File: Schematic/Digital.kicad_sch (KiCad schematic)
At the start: 19 parts, among them U801 74HC165, U802 74HC165, U803 74HC165, U804 74HC165, U805 74HC595, U806 ESP32-S3-DevKitC, U808 MCP42010, U809 MCP42010, U810 MCP42010, U811 MCP42010

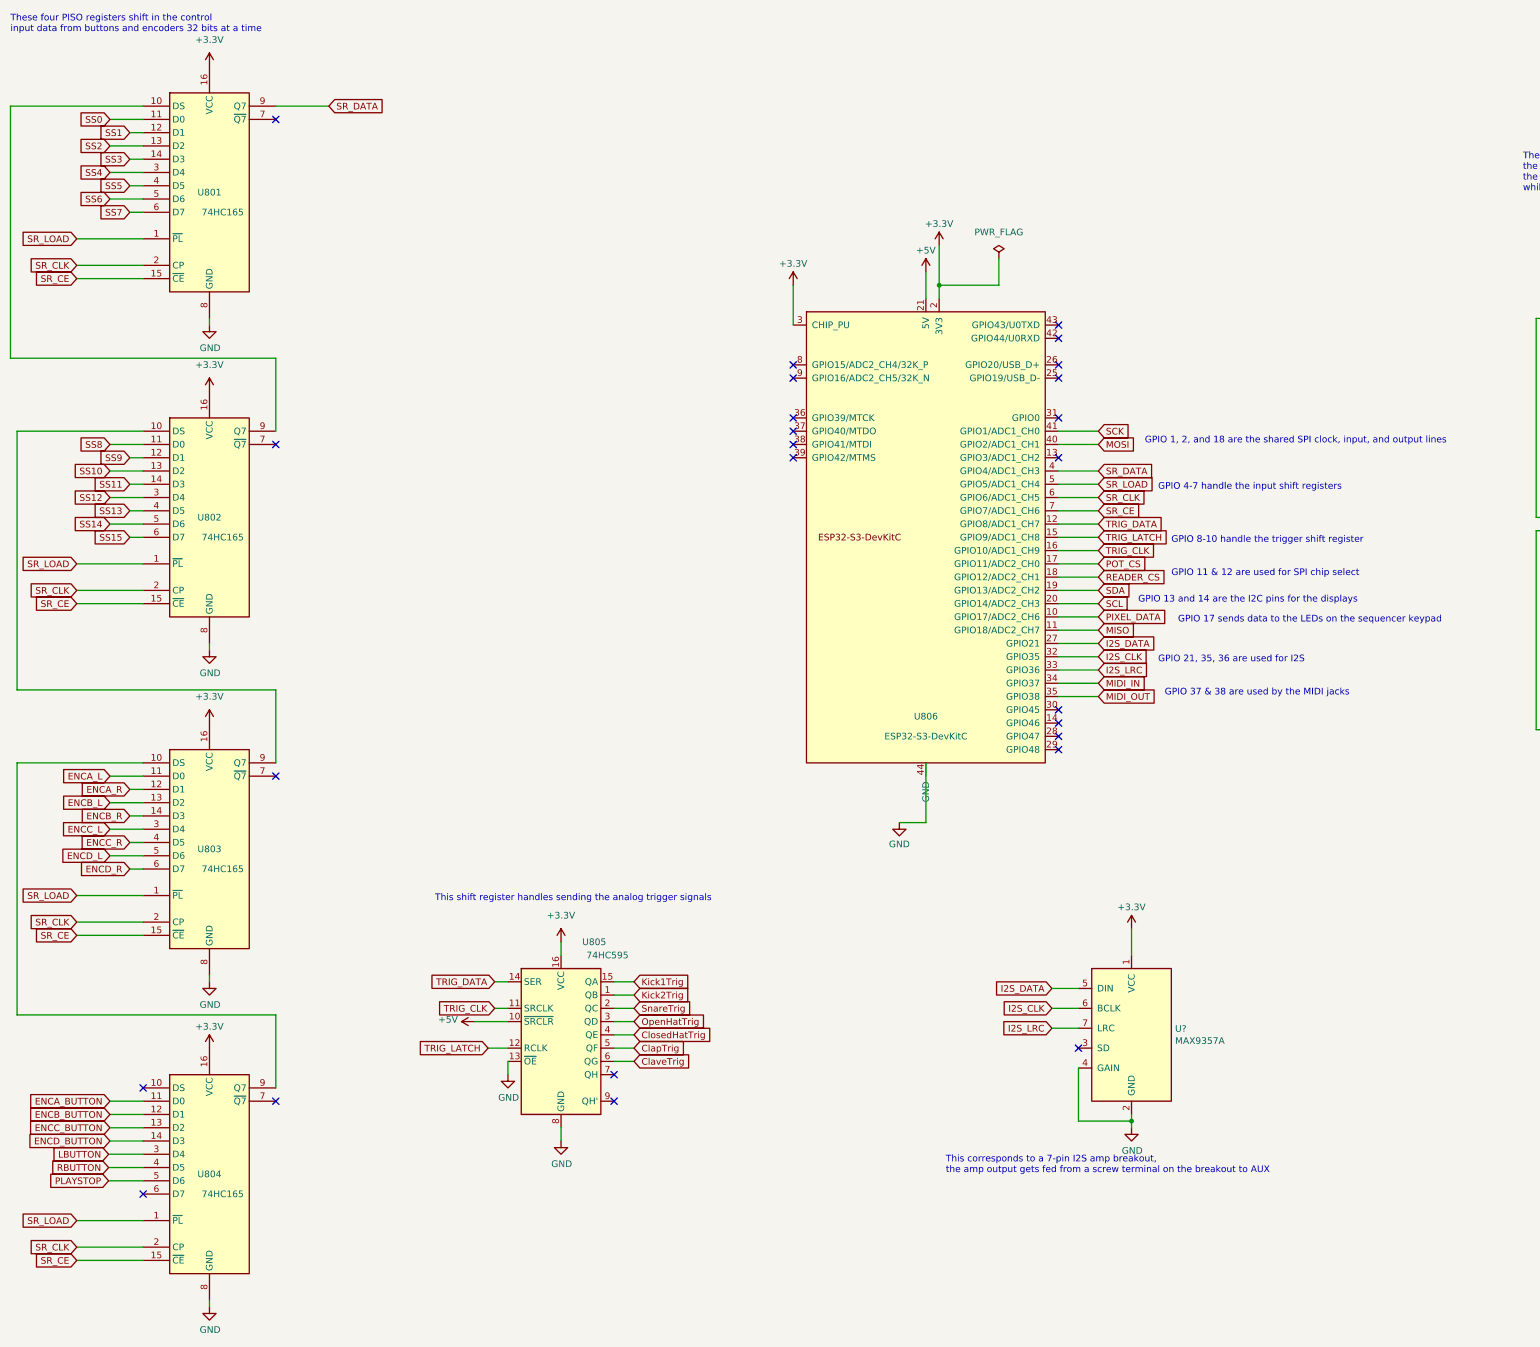
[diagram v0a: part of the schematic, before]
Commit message: cleansing fire
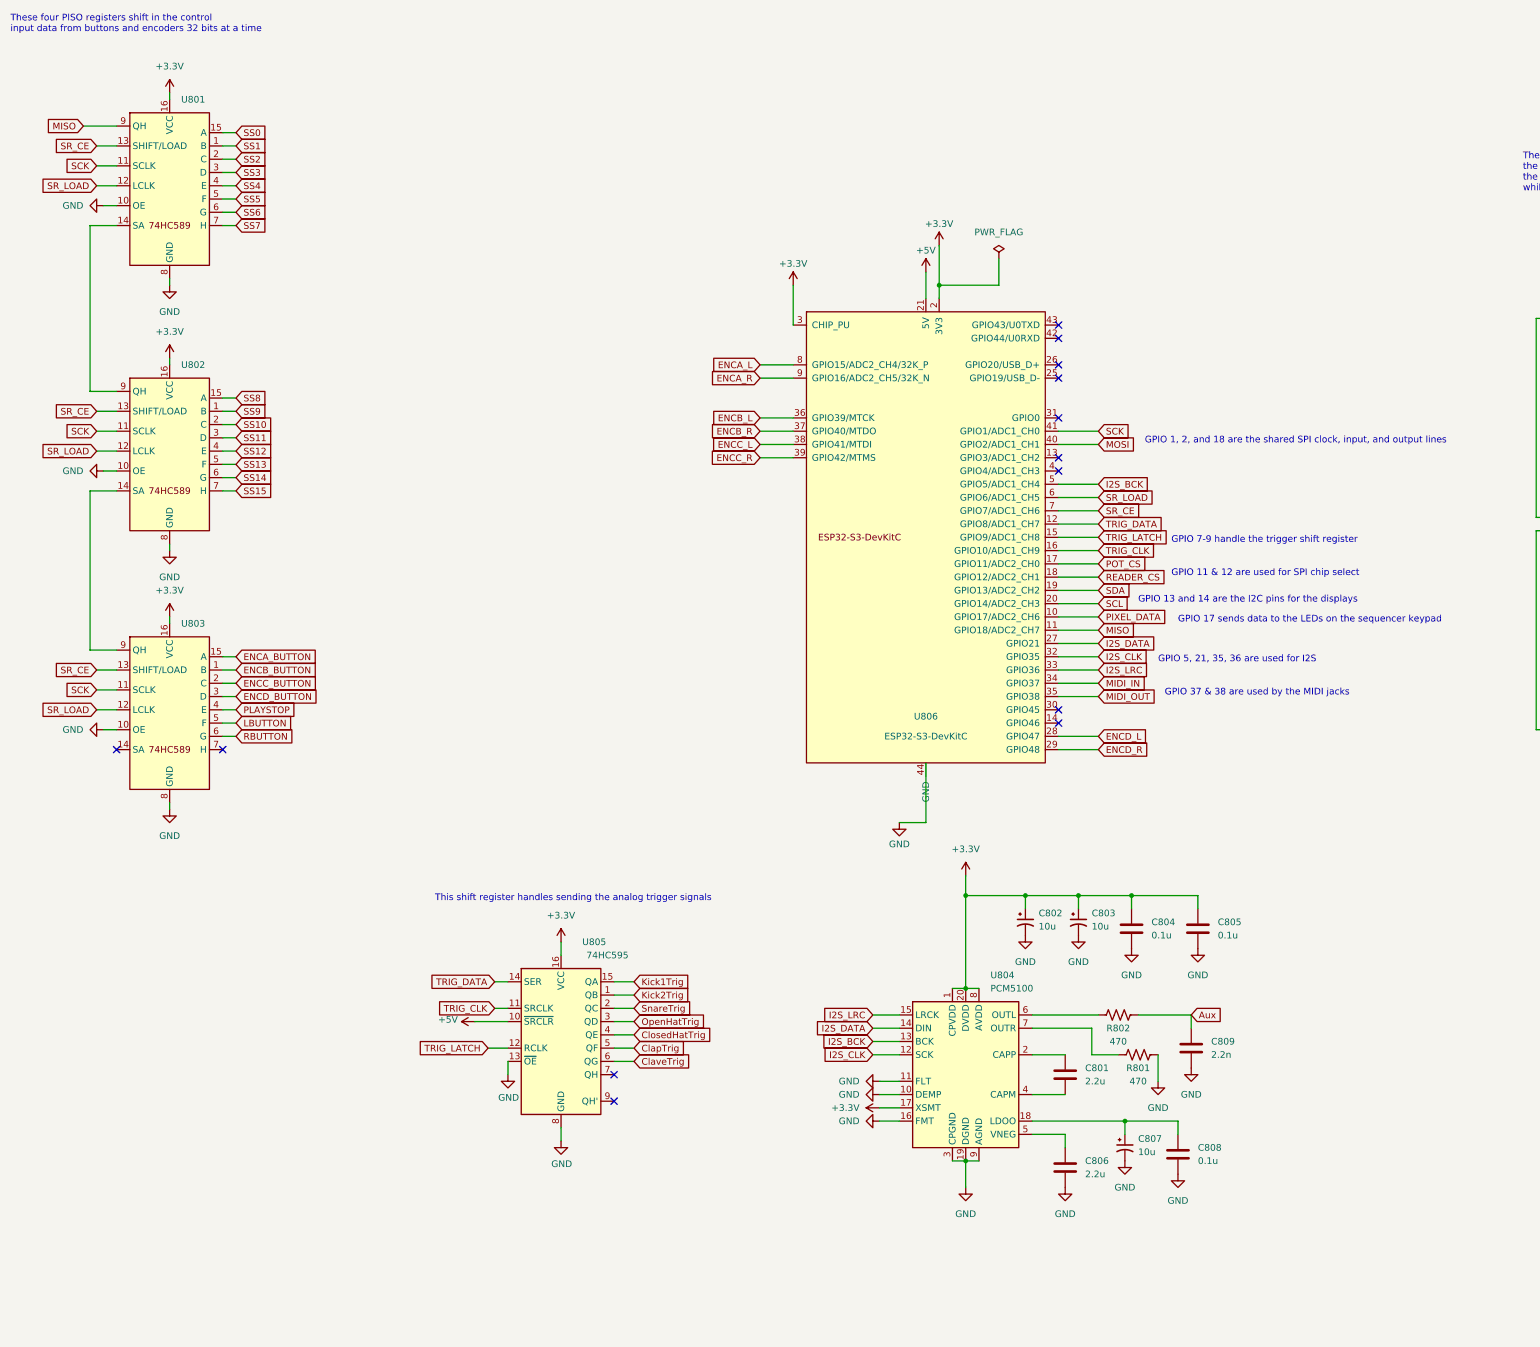
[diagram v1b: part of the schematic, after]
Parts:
- removed U801, U802, U803, U804: 74HC165, Package_DIP:DIP-16_W7.62mm, symbol 74xx:74HC165
- removed U?: MAX9357A, Connector_PinHeader_2.54mm:PinHeader_1x07_P2.54mm_Vertical, symbol ESP808-rescue:MAX9357A-Audio
- added C801, C806: 2.2u, Capacitor_THT:C_Disc_D4.7mm_W2.5mm_P5.00mm, symbol Device:C
- added C802, C803, C807: 10u, Capacitor_THT:CP_Radial_D5.0mm_P2.00mm, symbol Device:C_Polarized_Small_US
- added C804, C805, C808: 0.1u, Capacitor_THT:C_Disc_D4.7mm_W2.5mm_P5.00mm, symbol Device:C
- added C809: 2.2n, Capacitor_THT:C_Disc_D4.7mm_W2.5mm_P5.00mm, symbol Device:C
- added R801, R802: 470, PCM_Resistor_THT_AKL:R_Axial_DIN0207_L6.3mm_D2.5mm_P7.62mm_Horizontal, symbol Device:R_US
- added U801, U802, U803: ~, Package_SO:SO-16_3.9x9.9mm_P1.27mm, symbol 74xx:74HC589
- added U804: PCM5100, Package_SO:TSSOP-20_4.4x6.5mm_P0.65mm, symbol Audio:PCM5100
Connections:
- net SR_CLK is gone; now on net SR_LOAD: U806.6 (GPIO6/ADC1_CH5)
- net +3.3V: now also C802.1, C803.1, C804.1, C805.1, U801.16 (VCC), U802.16 (VCC), U803.16 (VCC), U804.1 (CPVDD), U804.17 (XSMT), U804.20 (DVDD), U804.8 (AVDD)
- net Aux: now also C809.1, R802.2
- net ENCA_BUTTON: now also U803.15 (A)
- net ENCA_L: now also U806.8 (GPIO15/ADC2_CH4/32K_P)
- net ENCA_R: now also U806.9 (GPIO16/ADC2_CH5/32K_N)
- net ENCB_BUTTON: now also U803.1 (B)
- net ENCB_L: now also U806.36 (GPIO39/MTCK)
- net ENCB_R: now also U806.37 (GPIO40/MTDO)
- net ENCC_BUTTON: now also U803.2 (C)
- net ENCC_L: now also U806.38 (GPIO41/MTDI)
- net ENCC_R: now also U806.39 (GPIO42/MTMS)
- net ENCD_BUTTON: now also U803.3 (D)
- net ENCD_L: now also U806.28 (GPIO47)
- net ENCD_R: now also U806.29 (GPIO48)
- net GND: now also C802.2, C803.2, C804.2, C805.2, C806.2, C807.2, C808.2, C809.2, R801.2, U801.10 (OE), U801.8 (GND), U802.10 (OE), U802.8 (GND), U803.10 (OE), U803.8 (GND), U804.10 (DEMP), U804.11 (FLT), U804.16 (FMT), U804.19 (DGND), U804.3 (CPGND), U804.9 (AGND)
- net I2S_CLK: now also U804.12 (SCK)
- net I2S_DATA: now also U804.14 (DIN)
- net I2S_LRC: now also U804.15 (LRCK)
- net LBUTTON: now also U803.5 (F)
- net MISO: now also U801.9 (QH)
- net PLAYSTOP: now also U803.4 (E)
- net RBUTTON: now also U803.6 (G)
- net SCK: now also U801.11 (SCLK), U802.11 (SCLK), U803.11 (SCLK)
- net SR_CE: now also U801.13 (SHIFT/LOAD), U802.13 (SHIFT/LOAD), U803.13 (SHIFT/LOAD)
- net SR_LOAD: now also U801.12 (LCLK), U802.12 (LCLK), U803.12 (LCLK); no longer U806.5 (GPIO5/ADC1_CH4)
- net SS0: now also U801.15 (A)
- net SS1: now also U801.1 (B)
- net SS10: now also U802.2 (C)
- net SS11: now also U802.3 (D)
- net SS12: now also U802.4 (E)
- net SS13: now also U802.5 (F)
- net SS14: now also U802.6 (G)
- net SS15: now also U802.7 (H)
- net SS2: now also U801.2 (C)
- net SS3: now also U801.3 (D)
- net SS4: now also U801.4 (E)
- net SS5: now also U801.5 (F)
- net SS6: now also U801.6 (G)
- net SS7: now also U801.7 (H)
- net SS8: now also U802.15 (A)
- net SS9: now also U802.1 (B)
- net SR_DATA: no longer names the net of U806.4 (GPIO4/ADC1_CH3)
- new net: R802.1, U804.6 (OUTL)
- new net: C806.1, U804.5 (VNEG)
- new net: C807.1, C808.1, U804.18 (LDOO)
- new net: C801.1, U804.2 (CAPP)
- new net: C801.2, U804.4 (CAPM)
- new net: R801.1, U804.7 (OUTR)
- new net: U802.14 (SA), U803.9 (QH)
- new net: U801.14 (SA), U802.9 (QH)
- new net I2S_BCK: U804.13 (BCK), U806.5 (GPIO5/ADC1_CH4)
- no-connect marks 26 -> 14
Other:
- note added: "GPIO 5, 21, 35, 36 are used for I2S"
- note added: "GPIO 7-9 handle the trigger shift register"
- note removed: "GPIO 21, 35, 36 are used for I2S"
- note removed: "GPIO 4-7 handle the input shift registers"
- note removed: "GPIO 8-10 handle the trigger shift register"
- note removed: "This corresponds to a 7-pin I2S amp breakout, the amp output gets fed from a screw terminal on the breakout to AUX"
